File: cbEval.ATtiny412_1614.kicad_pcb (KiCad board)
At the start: 2 copper layers, 35 x 109 mm, 59 parts, among them J1 Bergstik-II_3, J11 Bergstik-II_3, J12 Bergstik-II_3, J13 Bergstik-II_6, J14 Bergstik-II_6, J15 Bergstik-II_6, J16 Bergstik-II_3, J17 Bergstik-II_6, J18 Bergstik-II_3, J19 Bergstik-II_6, J2 Bergstik-II_6, J20 Bergstik-II_3, J21 Bergstik-II_3, J22 Bergstik-II_2, J23 Bergstik-II_2, J3 Header.Hor.2x8.9-103326-0-08, J4 Header.Hor.2x8.9-103326-0-08, J5 Socket.Hor.2x8.1-5535512-8, J6 Socket.Hor.2x8.1-5535512-8, J7 Bergstik-II_3, J8 Bergstik-II_2, U1 ATtiny412-SSFR, U2 ATtiny1614-SSFR

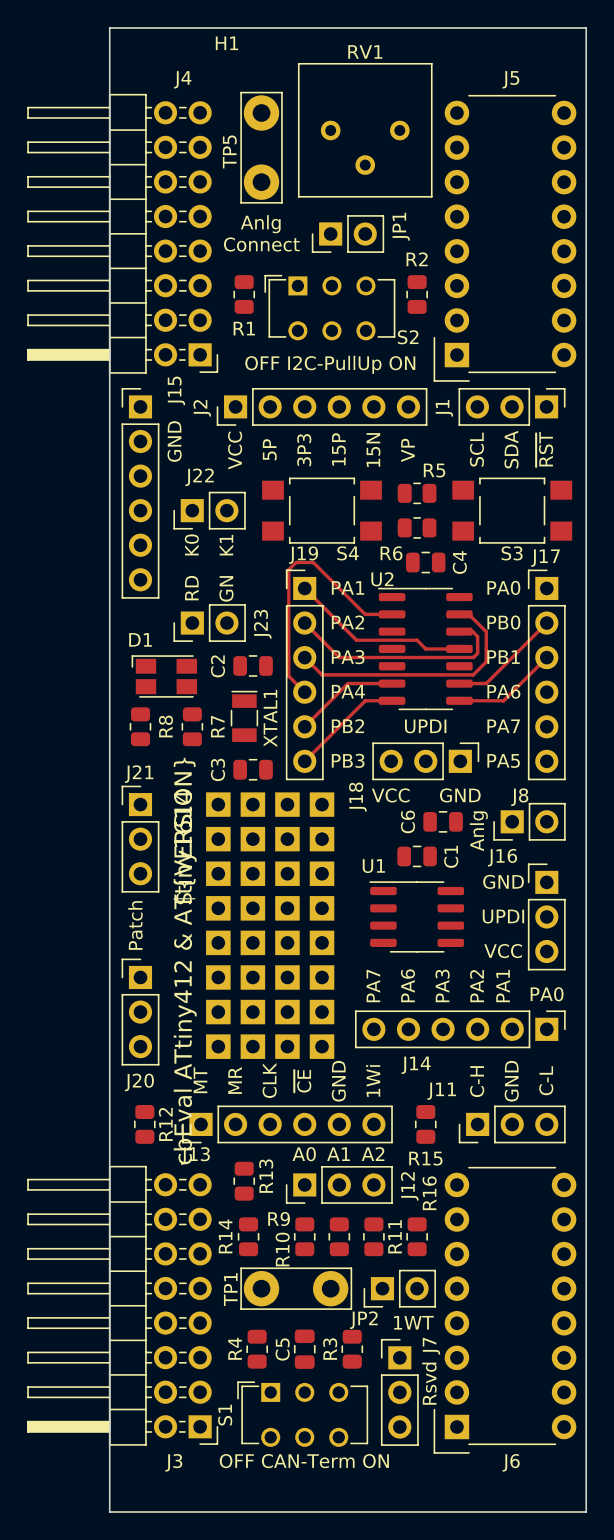
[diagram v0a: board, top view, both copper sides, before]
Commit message: alle Verbindungen layoutet
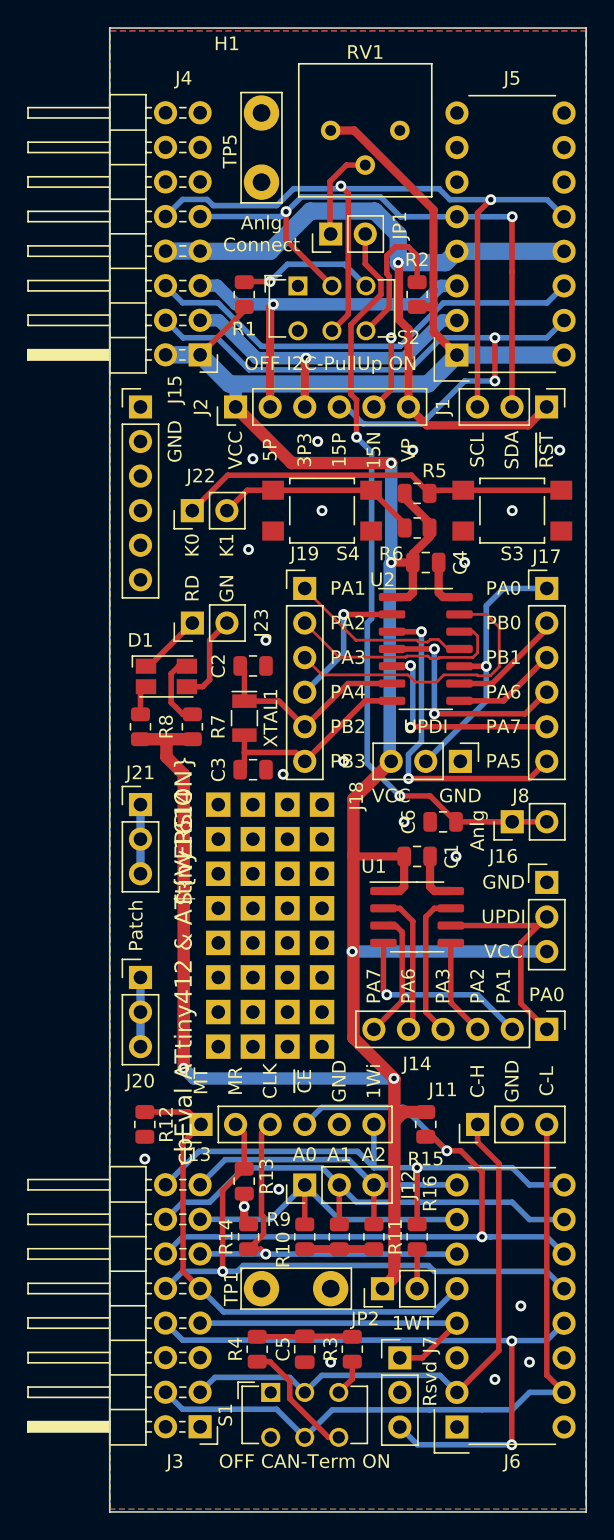
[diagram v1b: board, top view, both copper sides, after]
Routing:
- net VCC: track 0.00 -> 217.7 mm, vias 0 -> 5
- net /I2C-SCL: track 0.00 -> 58.3 mm, vias 0 -> 2
- net Net-(C6-Pad1): track 0.00 -> 56.0 mm, vias 0 -> 2
- net +VDC: track 0.00 -> 55.8 mm, vias 0 -> 1
- net /SPI-~{CE}: track 0.00 -> 52.6 mm, vias 0 -> 2
- net /CAN-L: track 0.00 -> 52.2 mm
- net +15V: track 0.00 -> 48.7 mm, vias 0 -> 2
- net /Reserved1: track 0.00 -> 46.8 mm, vias 0 -> 2
- net /I2C-SDA: track 0.00 -> 44.9 mm, vias 0 -> 2
- net /CAN-H: track 0.00 -> 42.4 mm
- net /SPI-MRST: track 0.00 -> 42.4 mm, vias 0 -> 1
- net -15V: track 0.00 -> 39.2 mm, vias 0 -> 1
- net /One-Wire: track 0.00 -> 38.7 mm, vias 0 -> 1
- net /SPI-MTSR: track 0.00 -> 37.9 mm
- net /SPI-ADR1: track 0.00 -> 35.3 mm
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- added copper zone on B.Cu, net GND
- added copper zone on F.Cu, net GND
